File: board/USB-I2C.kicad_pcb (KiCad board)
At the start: 2 copper layers, 44 x 18 mm, 17 parts, among them J1 USB_OTG, J2 Conn_01x06, U1 SPX3819, U2 STM32F042K4Tx, X1 I2C-6P, X2 I2C, X3 SWD

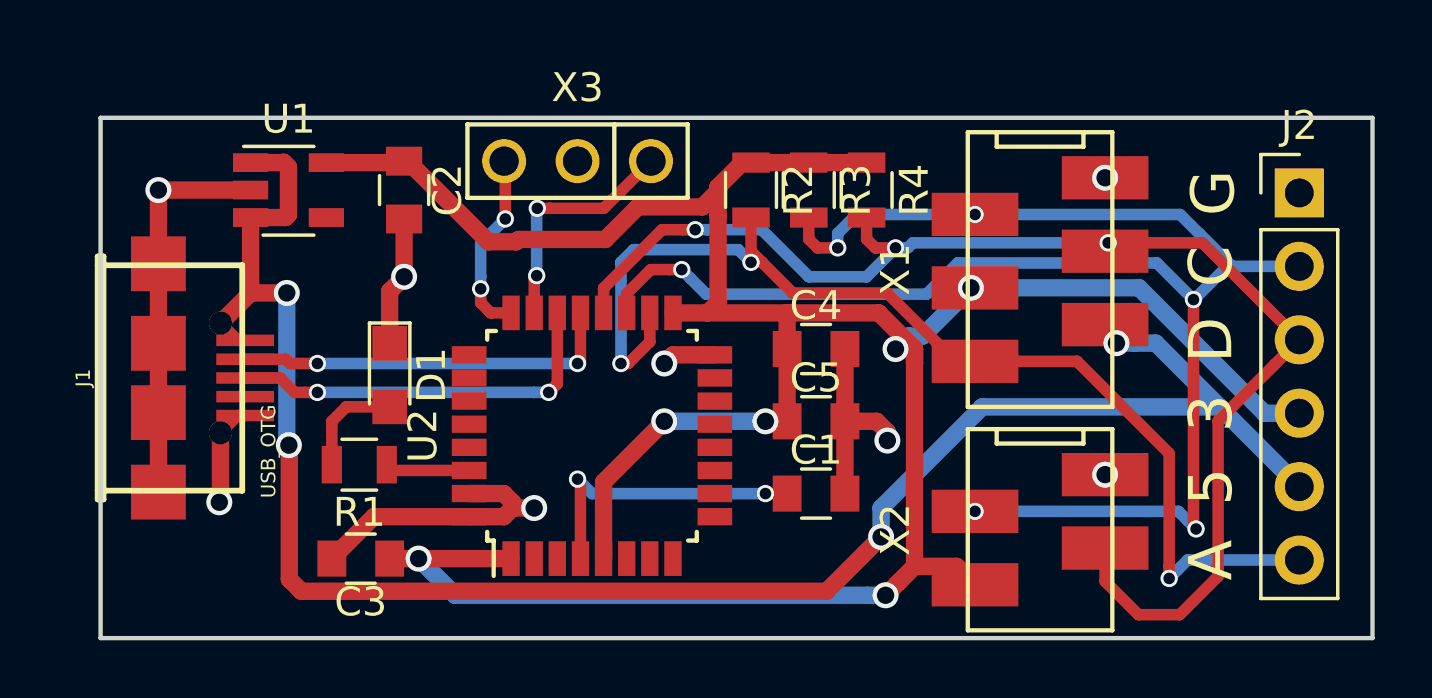
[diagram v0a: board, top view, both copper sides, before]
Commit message: WIP
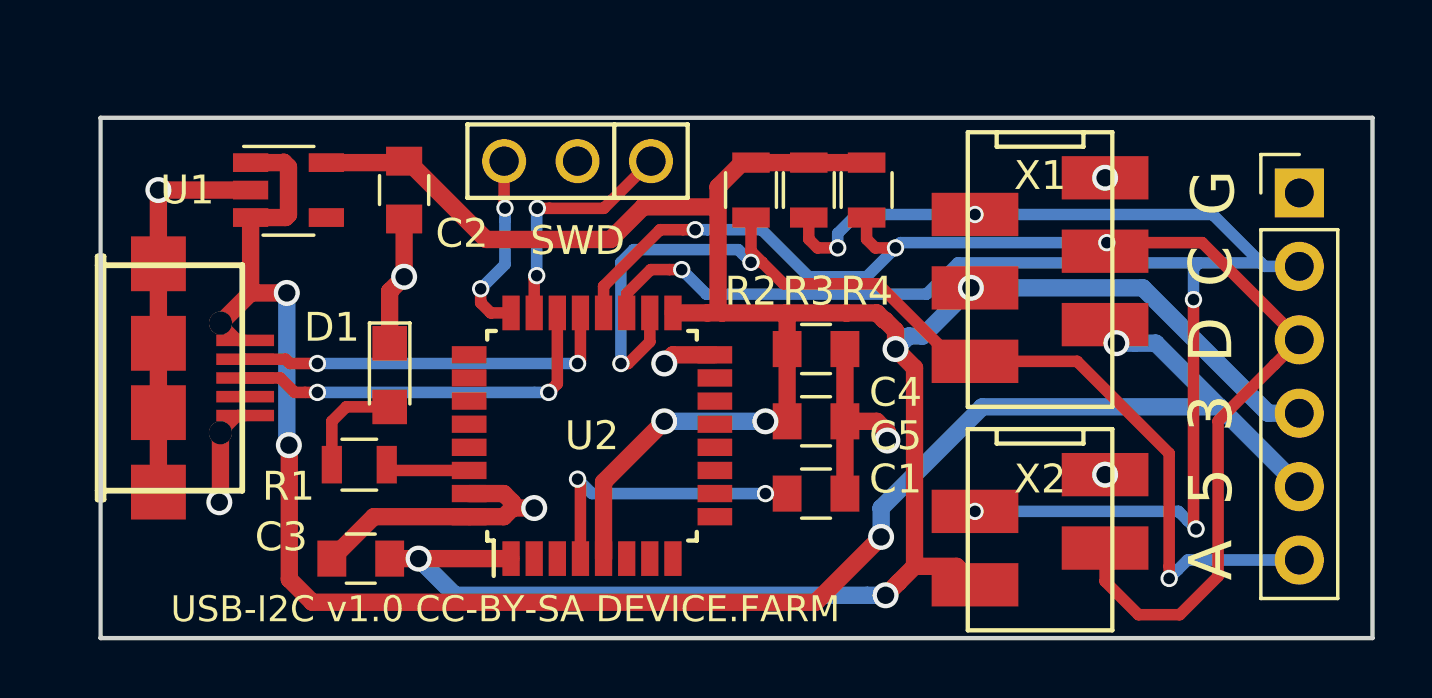
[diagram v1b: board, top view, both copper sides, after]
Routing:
- net +3V3: track 98.3 -> 96.4 mm
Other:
- board text added: "SWD"
- board text added: "USB-I2C v1.0 CC-BY-SA DEVICE.FARM"
